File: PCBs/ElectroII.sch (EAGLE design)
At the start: 37 parts, among them J1 U.FL-R-SMT(01), T1 VIN, T2 VBAT, T3 GND, T4 5V, T5 VCC, T6 ANT, U1 RFM95W-868S2, U2 TPS61090RSAR

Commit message: More board shuffling
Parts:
- added R7, R8: DNP, RTR Main Library:R-ALL_PACKAGESR1206
- added R9: 0.1 1/8w, RTR Main Library:R-ALL_PACKAGESR1206
- T4: value 5V -> BOOST
- T6: value ANT -> 5V
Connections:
- removed net I2C0_GPIO1: I2C0.6, U$1.GEN4/GPIO23
- new net CGND: R9.1
- new net SPI2_GPIO0: U$1.GEN5/GPIO24, U1.RESET
- new net SPI2_GPIO1: U$1.GEN4/GPIO23, U1.DIO0
- net 5V: now also T6.P$1
- net ANT: no longer T6.P$1
- net GND: now also R9.2
- net I2C0_GPIO0: no longer I2C0.4
- net I2C1_GPIO0: no longer U$1.GEN5/GPIO24
- net SCL: now also R8.1
- net SDA: now also R7.1
- net SPI0_GPIO0: no longer U1.RESET
- net SPI0_GPIO1: no longer U1.DIO0
- net VCC: now also R7.2, R8.2
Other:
- moved on the sheet: BRK0, C1, C2, C3, CN1, CR1, D1, F1, I2C0, I2C0_BRK, I2C1, I2C1_BRK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

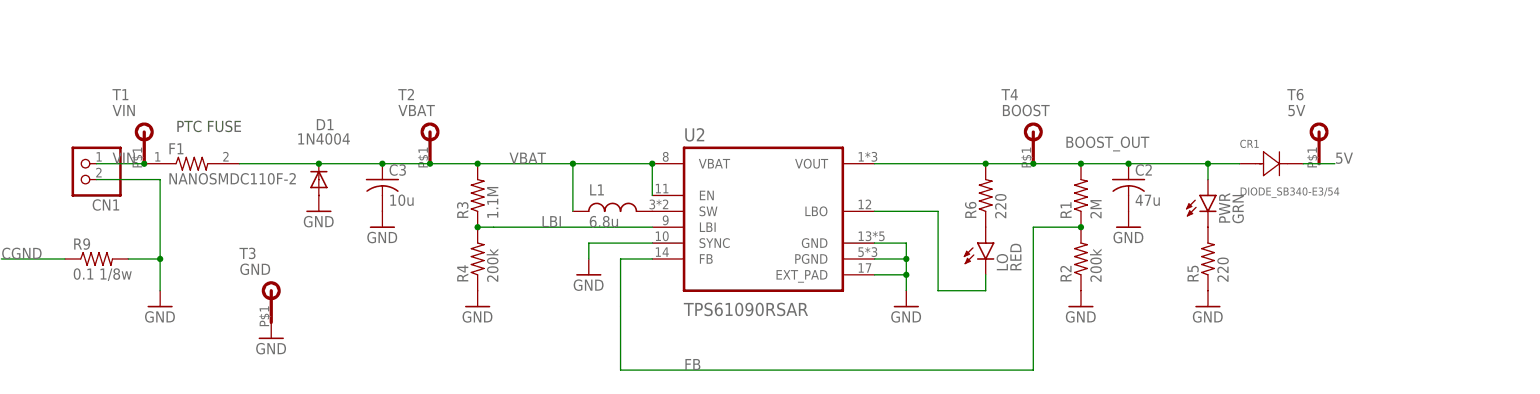
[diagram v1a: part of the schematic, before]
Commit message: more board shuffling
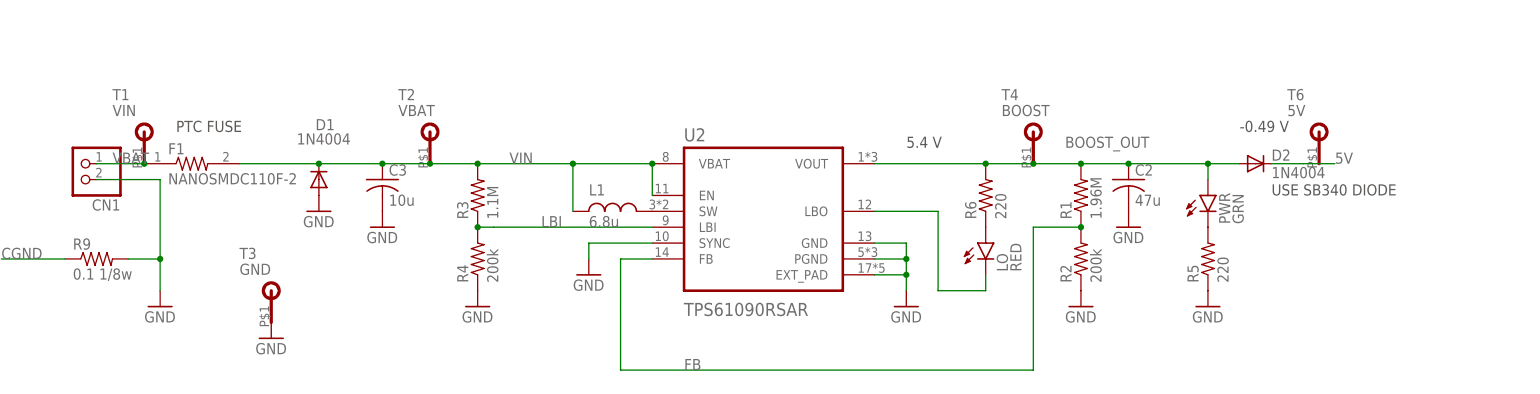
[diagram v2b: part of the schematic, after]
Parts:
- removed CR1: DIODE_SB340-E3/54, DIODE_SB340-E3-54:DIODE_SB340-E3/54
- added D2: 1N4004, adafruit:1N4004
- R1: value 2M -> 1.96M
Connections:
- net 5V: now also D2.C; no longer CR1.1
- net BOOST_OUT: now also D2.A; no longer CR1.2
- net VBAT: now also CN1.2, F1.1, T1.P$1; no longer C3.1, D1.C, F1.2, L1.1, R3.2, T2.P$1, U2.EN, U2.VBAT
- net VIN: now also C3.1, D1.C, F1.2, L1.1, R3.2, T2.P$1, U2.EN, U2.VBAT; no longer CN1.2, F1.1, T1.P$1
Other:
- note added: "-0.49 V"
- note added: "5.4 V"
- note added: "USE SB340 DIODE"
